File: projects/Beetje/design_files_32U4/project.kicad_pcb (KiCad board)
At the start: 2 copper layers, 25.4 x 25.4 mm, 27 parts, among them CON1 AVR-ISP-6, J2 Conn_01x06, J4 Conn_01x08, SW1 RESET, U1 ATMEGA32U4-AU, U2 MIC5225-3.3, X3 USB_OTG, Y1 8 Mhz

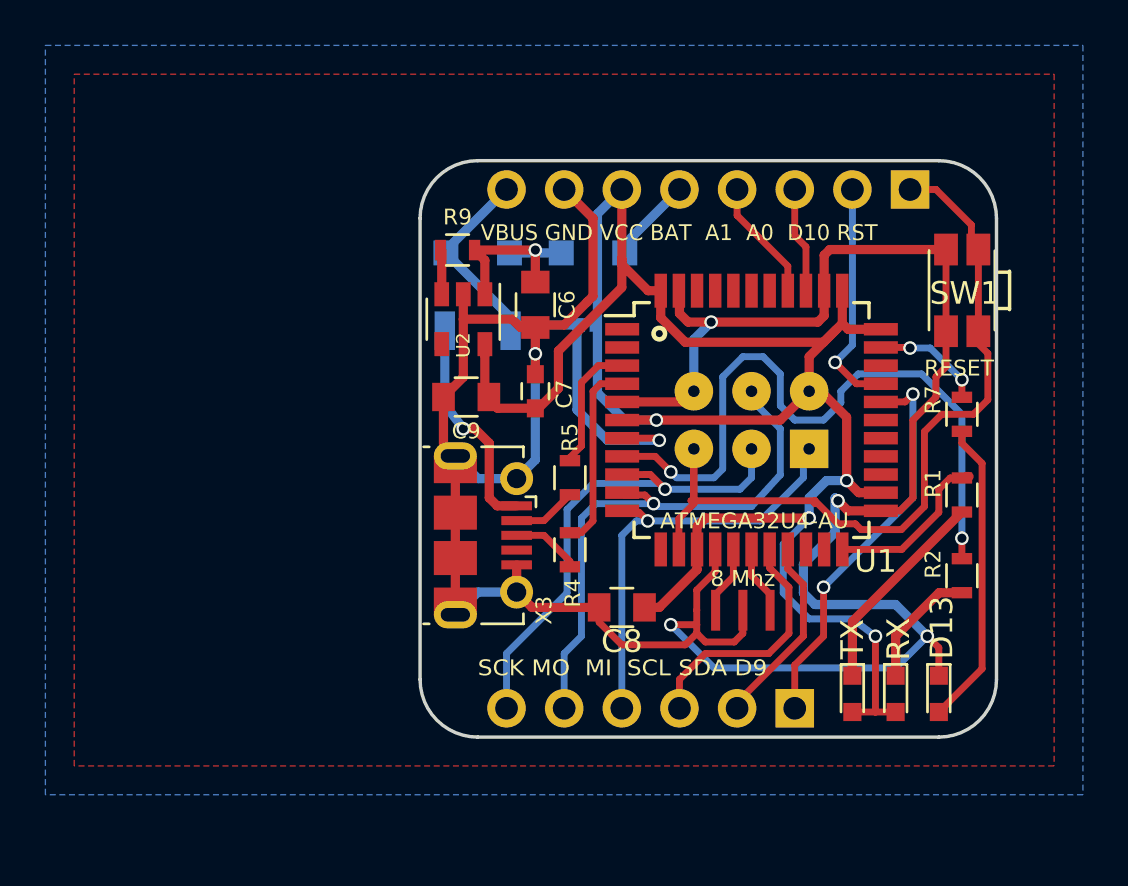
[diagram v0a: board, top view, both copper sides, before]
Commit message: Updates
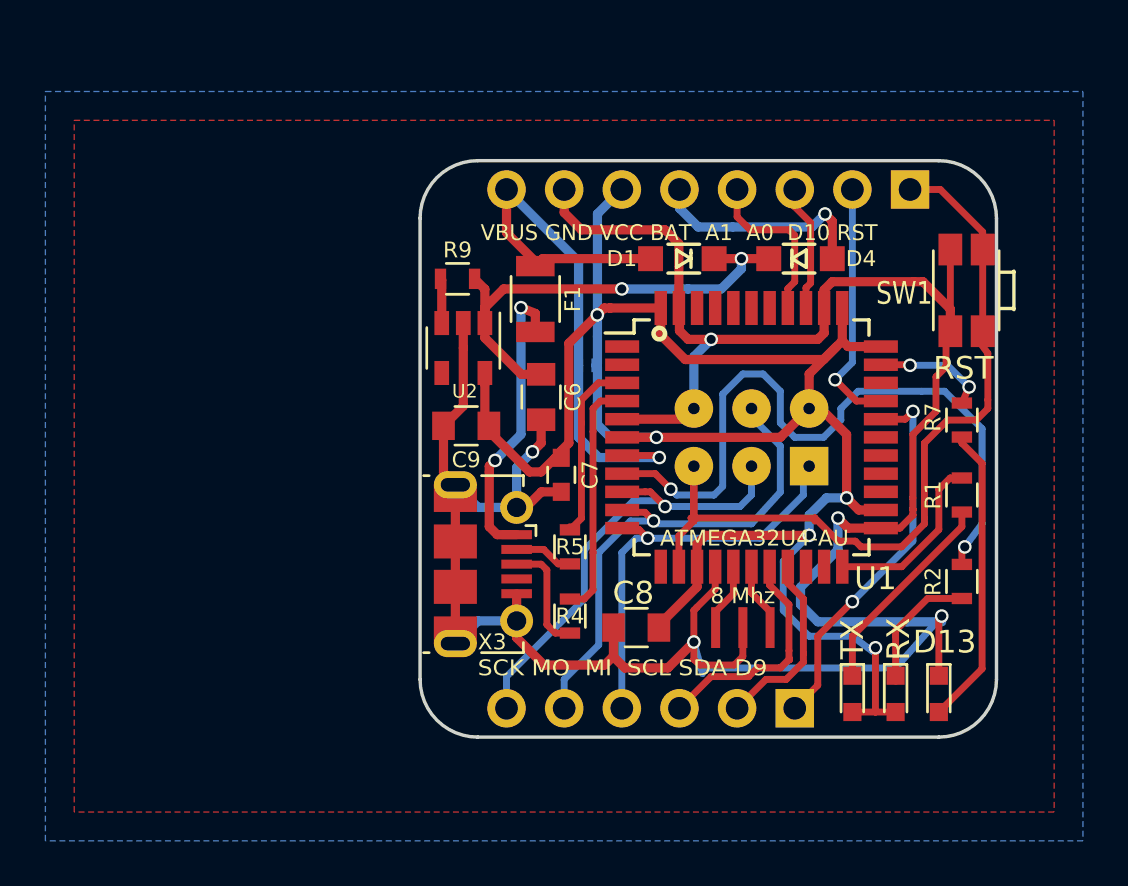
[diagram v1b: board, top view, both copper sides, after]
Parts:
- D1, D4, F1: moved to F.Cu
- SW1: value RESET -> RST
- moved D4 9.15 mm to (159.0, 90.7)
- moved D1 9.02 mm to (153.8, 90.7)
- moved C6 4.07 mm to (147.6, 96.8)
- moved C7 3.86 mm to (148.5, 100.2), turned to 270 degrees
- moved R5 3.05 mm to (148.8, 103.4)
- moved R4 2.92 mm to (148.8, 106.4)
- moved F1 2.90 mm to (147.3, 92.5), turned to 270 degrees
- moved JMP1 1.78 mm to (149.6, 95.4)
- moved C9 1.27 mm to (144.3, 98.0)
- moved R9 1.27 mm to (143.9, 91.6)
- moved U2 1.27 mm to (144.1, 94.6)
- moved X3 1.27 mm to (144.1, 104.1)
- moved C8 1.09 mm to (151.8, 106.9)
- moved CON1 0.76 mm to (159.4, 99.8)
- moved REF*** 0.76 mm to (158.6, 105.0)
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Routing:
- net /VHI: track 8.75 -> 21.5 mm, vias 1 -> 2
- net VBUS: track 21.2 -> 27.7 mm
- net +BATT: track 3.79 -> 9.92 mm, vias 0 -> 1
- net Net-(F1-Pad2): track 9.84 -> 13.1 mm, vias 1 -> 2
- net GND: track 123.5 -> 126.4 mm
- net /D-: track 5.75 -> 8.18 mm
- net /D+: track 8.37 -> 10.6 mm
- net /A1: track 5.39 -> 7.40 mm
- net Net-(R4-Pad2): track 3.06 -> 5.02 mm
- net /SCK: track 22.3 -> 20.5 mm
- net /MOSI: track 24.2 -> 22.6 mm
- net VCC: track 90.2 -> 88.9 mm, vias 4 -> 5
- net /~RESET: track 36.2 -> 37.3 mm
- net /A0: track 4.67 -> 5.60 mm
- net /MISO: track 19.4 -> 18.6 mm
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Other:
- board text added: "+ ISP -"
- board text added: "Rev 0.1 Aug 2018"
- board text removed: "- ISP +"
- board text removed: "Rev 0.0 Aug 2018"

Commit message: Updates
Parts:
- moved VAL 0.28 mm to (164.2, 97.9)
- moved REF*** 0.25 mm to (158.6, 105.3)
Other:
- board text added: "Beetje 32U4 Blok"
- board text added: "D9 SDA SCL MI MO SCK"
- board text added: "RST D10 A0 A0 BAT VCC GND VBUS"
- board text removed: "Beetje Blok 32U4"
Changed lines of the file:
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@@
-(kicad_pcb (version 4) (host pcbnew 4.0.6)
+(kicad_pcb (version 4) (host pcbnew 4.0.7)
   (general
     (links 77)
@@
     (area 142.164999 86.284999 167.715001 111.835001)
     (thickness 1.6)
-    (drawings 19)
+    (drawings 21)
     (tracks 416)
     (zones 0)
@@
     (34 B.Paste user)
     (35 F.Paste user)
-    (36 B.SilkS user hide)
+    (36 B.SilkS user)
     (37 F.SilkS user)
     (38 B.Mask user)
@@
     (44 Edge.Cuts user)
     (45 Margin user)
-    (46 B.CrtYd user)
+    (46 B.CrtYd user hide)
     (47 F.CrtYd user)
     (48 B.Fab user hide)
@@
   )
   (setup
-    (last_trace_width 0.3048)
+    (last_trace_width 0.25)
     (user_trace_width 0.3048)
     (user_trace_width 0.4064)
@@
     (pad 1 smd rect (at -1.8 -0.7 90) (size 1.4 1.05) (layers F.Cu F.Paste F.Mask)
       (net 1 GND))
-    (model ${KISYS3DMOD}/Buttons_Switches_SMD.3dshapes/SW_SPST_KMR2.wrl
-      (at (xyz 0 0 0))
-      (scale (xyz 1 1 1))
-      (rotate (xyz 0 0 0))
-    )
-    (model "C:/Users/Maker's Box/Downloads/3d_switch (1)/walter/switch/smd_push2.wrl"
-      (at (xyz 0 0 0))
-      (scale (xyz 1 1 1))
-      (rotate (xyz 0 0 0))
-    )
   )
   (module myFootPrints:MadeInOregonRev25 (layer F.Cu)
-    (at 164.084 98.171)
+    (at 164.211 97.917)
     (fp_text reference VAL (at 0 0) (layer F.SilkS) hide
       (effects (font (size 1.143 1.143) (thickness 0.1778)))
@@
   )
   (module footprints:KiCad-Logo2_8mm_SilkScreen (layer B.Cu)
-    (at 158.623 105.029 180)
+    (at 158.623 105.283 180)
     (descr "KiCad Logo")
     (tags "Logo KiCad")
@@
     )
   )
+  (gr_text "RST D10  A0  A0  BAT VCC GND VBUS" (at 164.719 89.535) (layer B.SilkS)
+    (effects (font (size 0.7 0.675) (thickness 0.16875)) (justify left mirror))
+  )
+  (gr_text "D9 SDA SCL  MI  MO SCK" (at 159.512 108.712) (layer B.SilkS)
+    (effects (font (size 0.7 0.75) (thickness 0.175)) (justify left mirror))
+  )
   (gr_text "Rev 0.1\nAug 2018" (at 148.463 104.013) (layer B.SilkS)
     (effects (font (size 0.75 0.75) (thickness 0.15)) (justify left mirror))
@@
     (arrow2b (pts (xy 167.64 81.280001) (xy 166.513496 81.866422)))
   )
-  (gr_text "+ ISP -" (at 156.845 94.234) (layer B.SilkS)
-    (effects (font (size 1.25 1.25) (thickness 0.3)) (justify mirror))
+  (gr_text "+ ISP -" (at 156.591 95.25) (layer B.SilkS)
+    (effects (font (size 1 1) (thickness 0.25)) (justify mirror))
   )
   (gr_circle (center 152.781 93.98) (end 152.781 93.726) (layer F.SilkS) (width 0.2))
-  (gr_text www.MakersBox.us (at 166.751 108.204) (layer B.SilkS)
+  (gr_text www.MakersBox.us (at 166.878 93.599) (layer B.SilkS)
     (effects (font (size 1.75 1.75) (thickness 0.3) italic) (justify left mirror))
   )
-  (gr_text "Beetje Blok\n32U4" (at 167.132 91.44) (layer B.SilkS)
+  (gr_text "Beetje 32U4 Blok\n" (at 167.132 91.44) (layer B.SilkS)
     (effects (font (size 1.75 1.75) (thickness 0.4) italic) (justify left mirror))
   )
@@
     (effects (font (size 0.7 0.75) (thickness 0.175)) (justify left))
   )
-  (segment (start 165.416 94.0655) (end 165.416 95.442) (width 0.3048) (layer F.Cu) (net 1) (status 400000))
+  (segment (start 165.416 94.0655) (end 165.416 95.442) (width 0.3048) (layer F.Cu) (net 1))
   (segment (start 164.973 95.885) (end 165.416 95.442) (width 0.3048) (layer F.Cu) (net 1))
   (segment (start 164.973 97.409) (end 164.973 95.885) (width 0.3048) (layer F.Cu) (net 1))
@@
   (segment (start 163.957 101.219) (end 163.957 98.425) (width 0.3048) (layer F.Cu) (net 1))
   (segment (start 163.957 101.219) (end 163.957 101.723802) (width 0.3048) (layer F.Cu) (net 1))
-  (segment (start 165.416 94.0655) (end 165.6065 93.875) (width 0.3048) (layer F.Cu) (net 1) (status C00000))
+  (segment (start 165.416 94.0655) (end 165.6065 93.875) (width 0.3048) (layer F.Cu) (net 1))
   (segment (start 163.997 91.694) (end 164.4015 91.694) (width 0.4064) (layer F.Cu) (net 1))
   (segment (start 160.045 92.05) (end 160.401 91.694) (width 0.4064) (layer F.Cu) (net 1))
   (segment (start 160.401 91.694) (end 163.997 91.694) (width 0.4064) (layer F.Cu) (net 1))
   (segment (start 160.045 92.852) (end 160.045 92.05) (width 0.4064) (layer F.Cu) (net 1))
-  (segment (start 165.6065 92.899) (end 165.6065 93.875) (width 0.4064) (layer F.Cu) (net 1) (status 800000))
+  (segment (start 165.6065 92.899) (end 165.6065 93.875) (width 0.4064) (layer F.Cu) (net 1))
   (segment (start 164.4015 91.694) (end 165.6065 92.899) (width 0.4064) (layer F.Cu) (net 1))
   (segment (start 163.957 101.981) (end 163.957 101.723802) (width 0.3048) (layer F.Cu) (net 1))
